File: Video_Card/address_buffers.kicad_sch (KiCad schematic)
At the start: 3 parts, among them U2 74FCT162244, U3 74FCT162244, U4 SN74AHCT1G32DBV

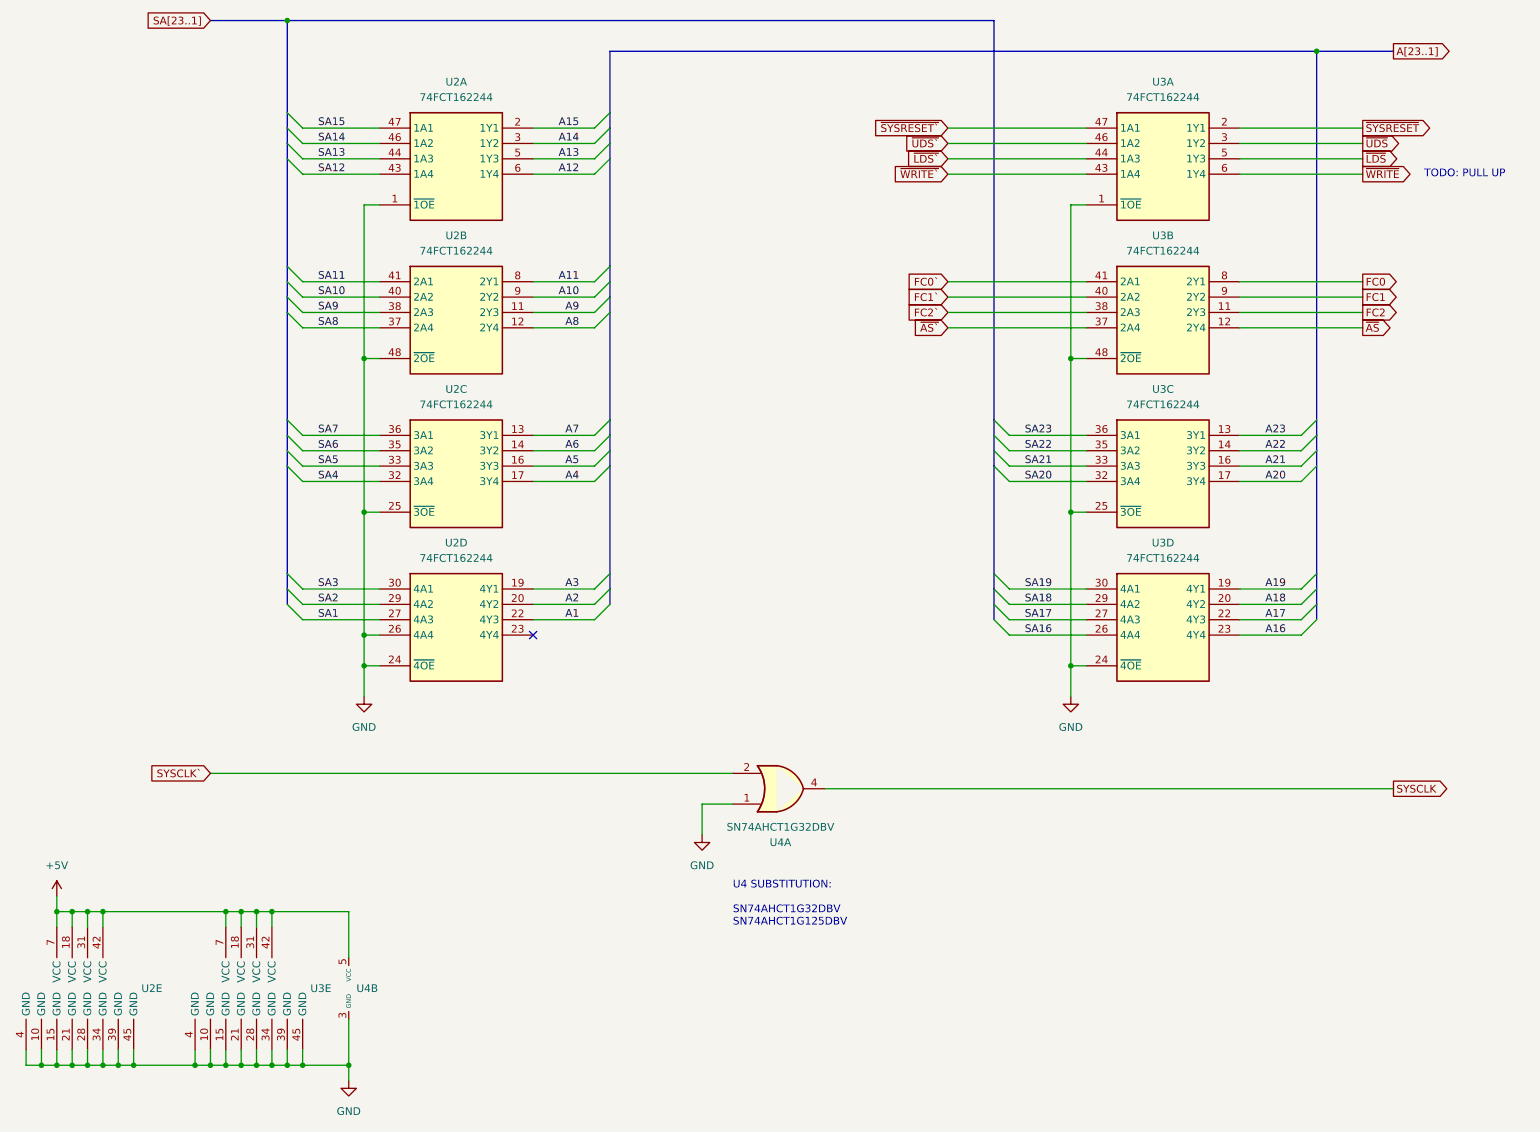
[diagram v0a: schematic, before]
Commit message: Final work for rev 1
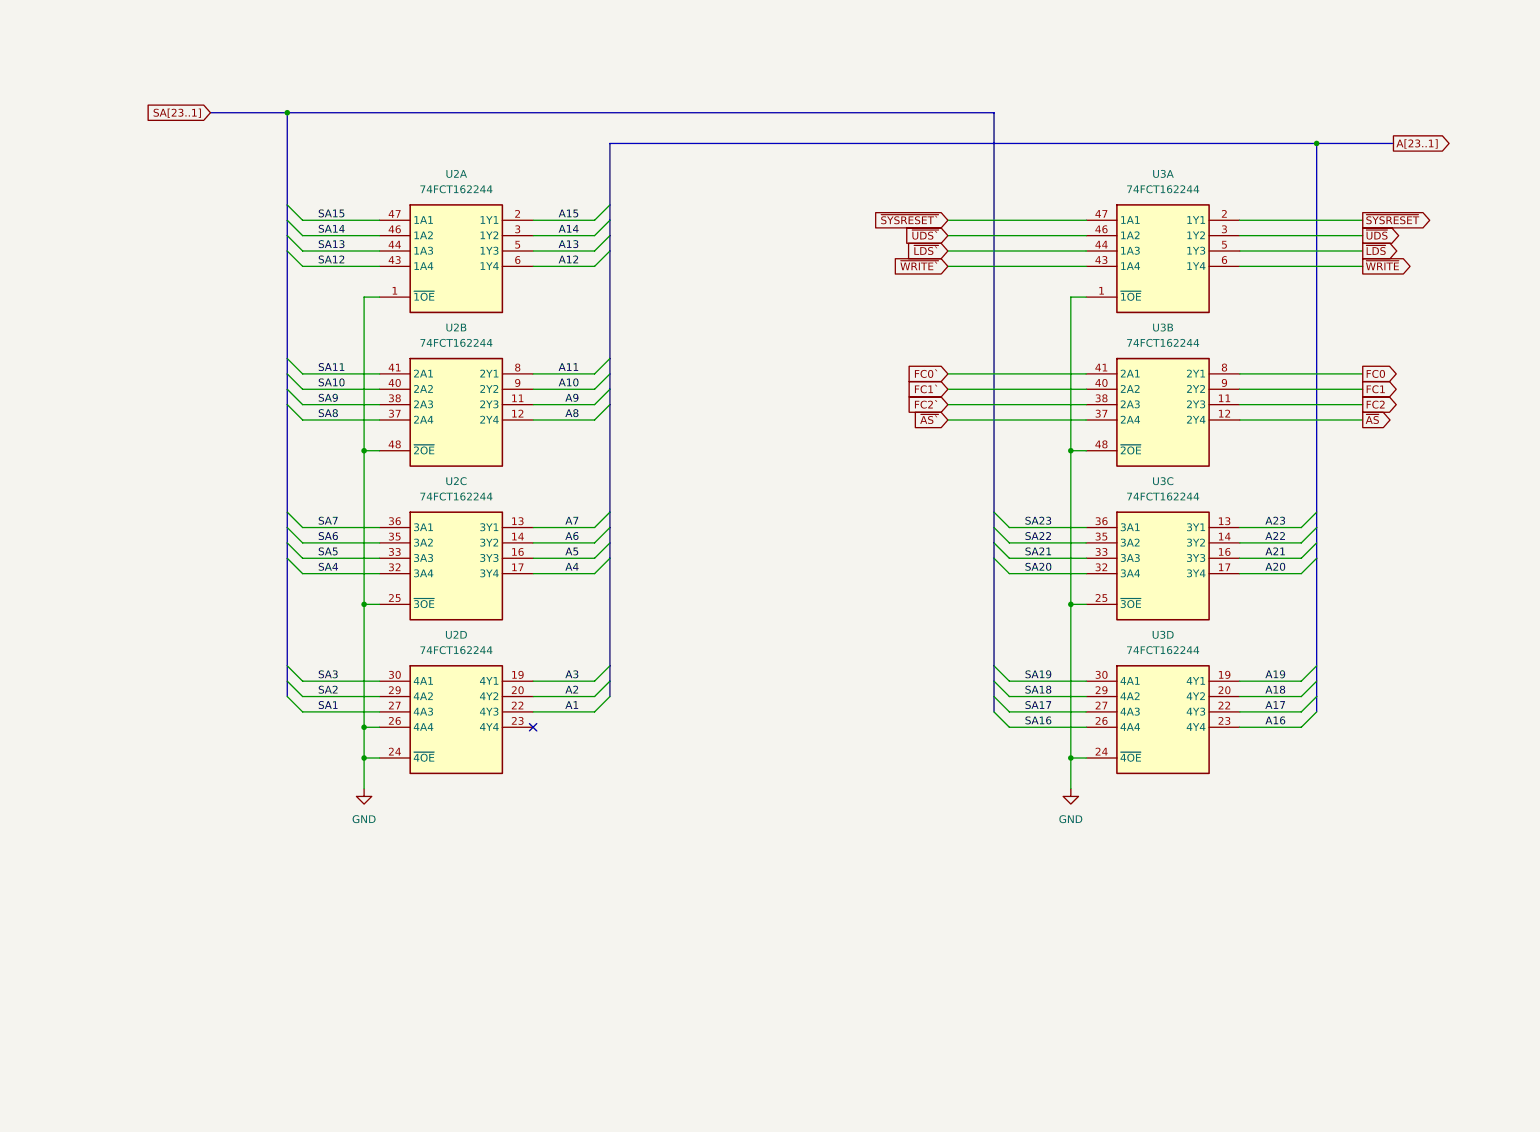
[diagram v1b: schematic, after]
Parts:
- removed unit 5 of U2
- removed unit 5 of U3
- removed U4: SN74AHCT1G32DBV, COMET_footprints:Package_SOT23-5, symbol COMET_symbols:74x1G32
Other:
- note removed: "TODO: PULL UP"
- note removed: "U4 SUBSTITUTION: SN74AHCT1G32DBV SN74AHCT1G125DBV"
- moved on the sheet: U2A, U2B, U2C, U2D, U3A, U3B, U3C, U3D
